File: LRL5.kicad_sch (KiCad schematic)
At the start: 30 parts, among them J1 POWER, J2 On/Off, J5 OUT, J6 MODE, Q1 BC549, U1 BA033CC0T, U2 NHD-C0220BIZ

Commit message: Added filled zone
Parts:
- J3, J4: footprint Connector_PinHeader_2.54mm:PinHeader_1x20_P2.54mm_Vertical -> Connector_PinHeader_2.54mm:PinHeader_1x20_P2.54mm_Vertical_SMD_Pin1Left
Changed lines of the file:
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@@
 			)
 		)
-		(property "Footprint" "Connector_PinHeader_2.54mm:PinHeader_1x20_P2.54mm_Vertical"
+		(property "Footprint" "Connector_PinHeader_2.54mm:PinHeader_1x20_P2.54mm_Vertical_SMD_Pin1Left"
 			(at 250.19 57.15 0)
 			(effects
@@
 			)
 		)
-		(property "Footprint" "Connector_PinHeader_2.54mm:PinHeader_1x20_P2.54mm_Vertical"
+		(property "Footprint" "Connector_PinHeader_2.54mm:PinHeader_1x20_P2.54mm_Vertical_SMD_Pin1Left"
 			(at 231.14 57.15 0)
 			(effects

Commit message: Some fixes
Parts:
- H1, H2, H3, H4: footprint MountingHole:MountingHole_2.5mm -> MountingHole:MountingHole_3.2mm_M3
- J2: footprint Connector_PinHeader_2.54mm:PinHeader_1x02_P2.54mm_Vertical -> Connector_PinHeader_2.54mm:PinHeader_1x02_P2.54mm_Vertical_SMD_Pin1Left
- J5: footprint Connector_PinHeader_2.54mm:PinHeader_1x03_P2.54mm_Vertical -> Connector_PinHeader_2.54mm:PinHeader_1x03_P2.54mm_Vertical_SMD_Pin1Left
- J6: footprint Connector_PinHeader_2.54mm:PinHeader_1x04_P2.54mm_Vertical -> Connector_PinHeader_2.54mm:PinHeader_1x04_P2.54mm_Vertical_SMD_Pin1Left
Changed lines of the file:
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@@
 			)
 		)
-		(property "Footprint" "MountingHole:MountingHole_2.5mm"
+		(property "Footprint" "MountingHole:MountingHole_3.2mm_M3"
 			(at 25.4 104.14 0)
 			(effects
@@
 			)
 		)
-		(property "Footprint" "Connector_PinHeader_2.54mm:PinHeader_1x02_P2.54mm_Vertical"
+		(property "Footprint" "Connector_PinHeader_2.54mm:PinHeader_1x02_P2.54mm_Vertical_SMD_Pin1Left"
 			(at 247.65 121.92 0)
 			(effects
@@
 			)
 		)
-		(property "Footprint" "MountingHole:MountingHole_2.5mm"
+		(property "Footprint" "MountingHole:MountingHole_3.2mm_M3"
 			(at 25.4 109.22 0)
 			(effects
@@
 			)
 		)
-		(property "Footprint" "MountingHole:MountingHole_2.5mm"
+		(property "Footprint" "MountingHole:MountingHole_3.2mm_M3"
 			(at 25.4 99.06 0)
 			(effects
@@
 			)
 		)
-		(property "Footprint" "MountingHole:MountingHole_2.5mm"
+		(property "Footprint" "MountingHole:MountingHole_3.2mm_M3"
 			(at 25.4 93.98 0)
 			(effects
@@
 			)
 		)
-		(property "Footprint" "Connector_PinHeader_2.54mm:PinHeader_1x04_P2.54mm_Vertical"
+		(property "Footprint" "Connector_PinHeader_2.54mm:PinHeader_1x04_P2.54mm_Vertical_SMD_Pin1Left"
 			(at 189.23 40.64 0)
 			(effects
@@
 			)
 		)
-		(property "Footprint" "Connector_PinHeader_2.54mm:PinHeader_1x03_P2.54mm_Vertical"
+		(property "Footprint" "Connector_PinHeader_2.54mm:PinHeader_1x03_P2.54mm_Vertical_SMD_Pin1Left"
 			(at 91.44 147.32 0)
 			(effects

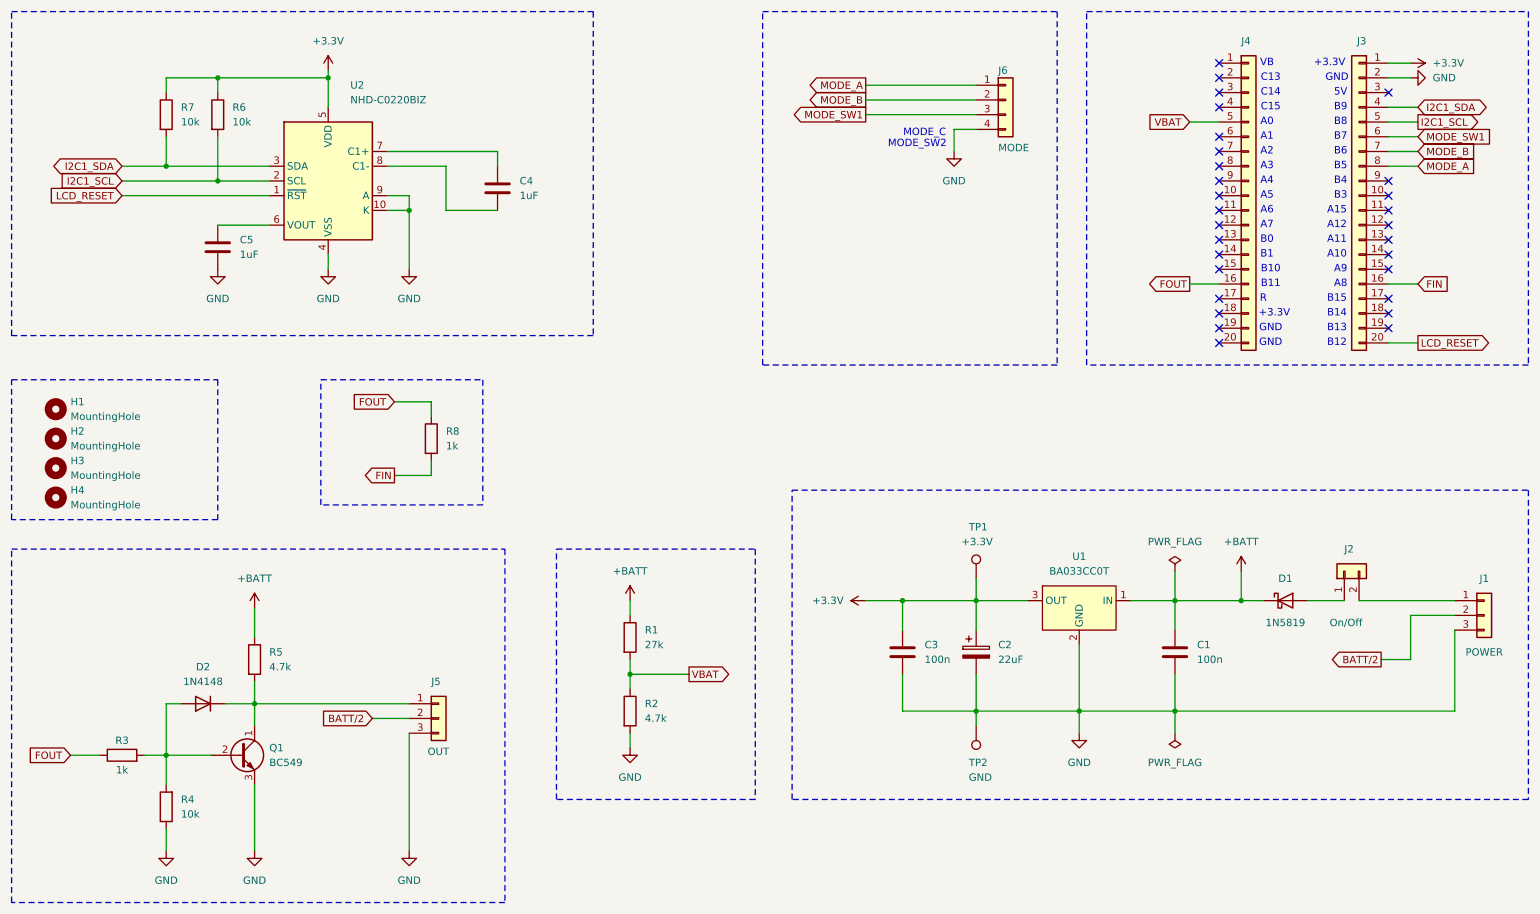
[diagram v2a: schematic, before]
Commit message: Some fixes 2
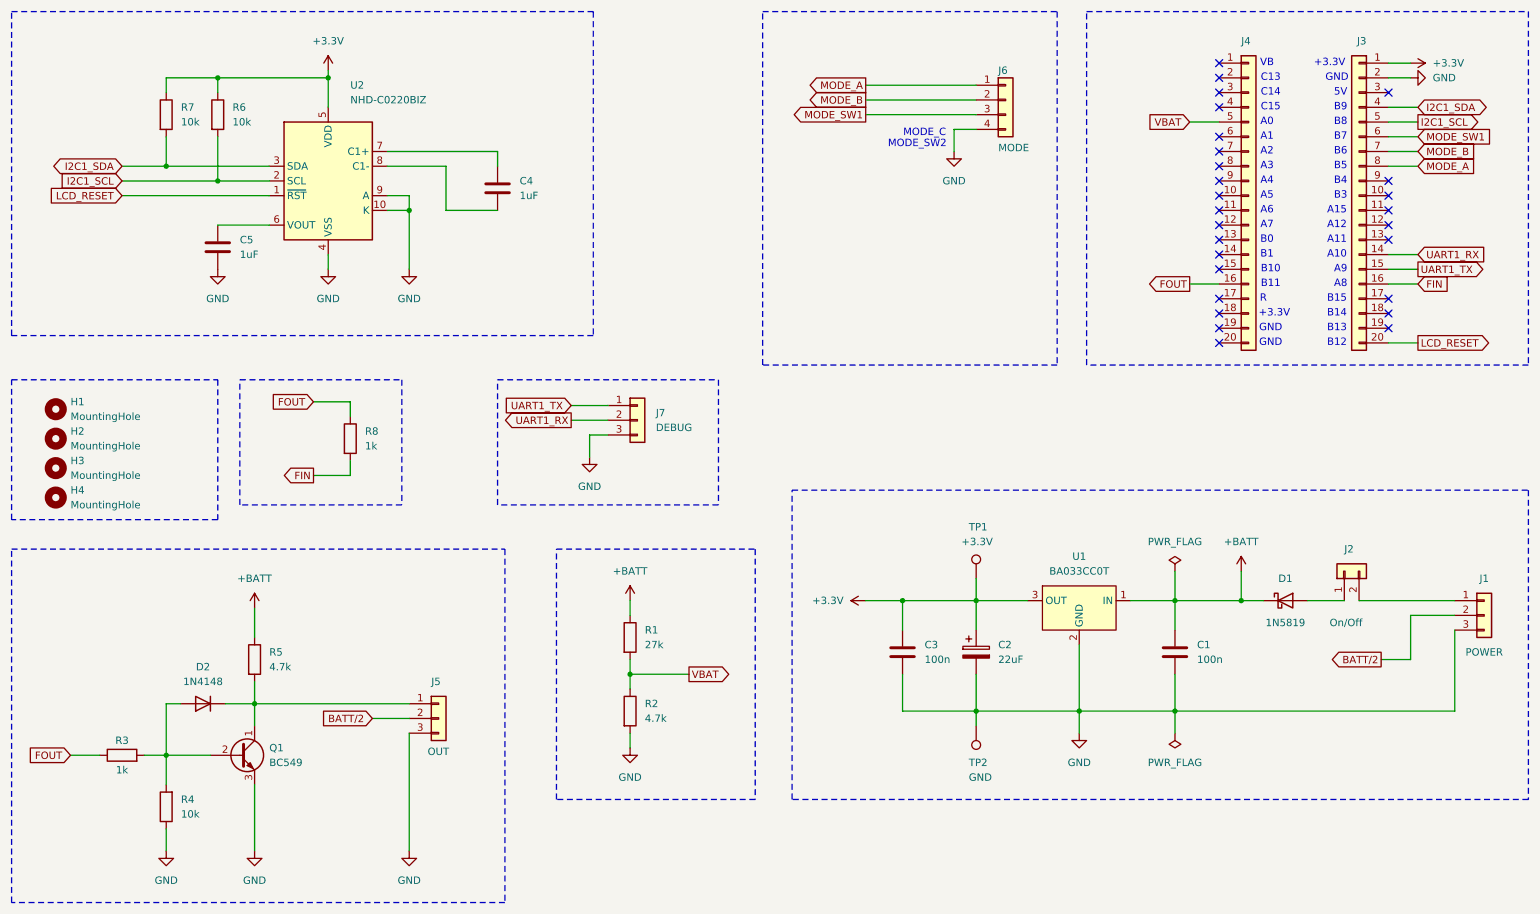
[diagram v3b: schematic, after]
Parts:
- added J7: DEBUG, Connector_PinHeader_2.54mm:PinHeader_1x03_P2.54mm_Vertical_SMD_Pin1Left, symbol Connector_Generic:Conn_01x03
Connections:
- net GND: now also J7.3 (Pin_3)
- net UART1_RX: now reaches J3.14 (Pin_14)
- net UART1_RX: now also J7.2 (Pin_2)
- net UART1_TX: now reaches J3.15 (Pin_15)
- net UART1_TX: now also J7.1 (Pin_1)
- no-connect marks 29 -> 27
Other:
- moved on the sheet: R8
